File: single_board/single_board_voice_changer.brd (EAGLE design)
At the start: 58.1 x 48.2 mm, 26 parts, among them U1 ATMEGA328P_PDIP

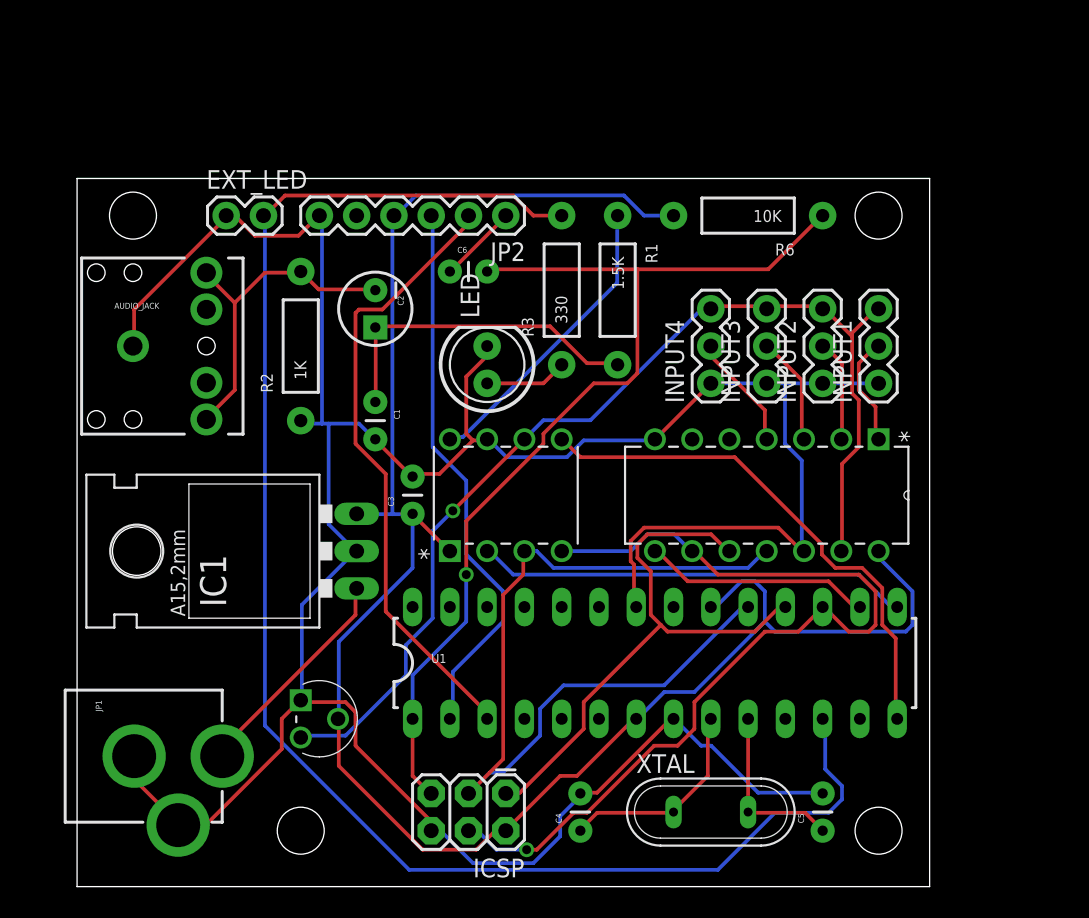
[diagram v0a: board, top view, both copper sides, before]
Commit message: board with no ground plane, 0
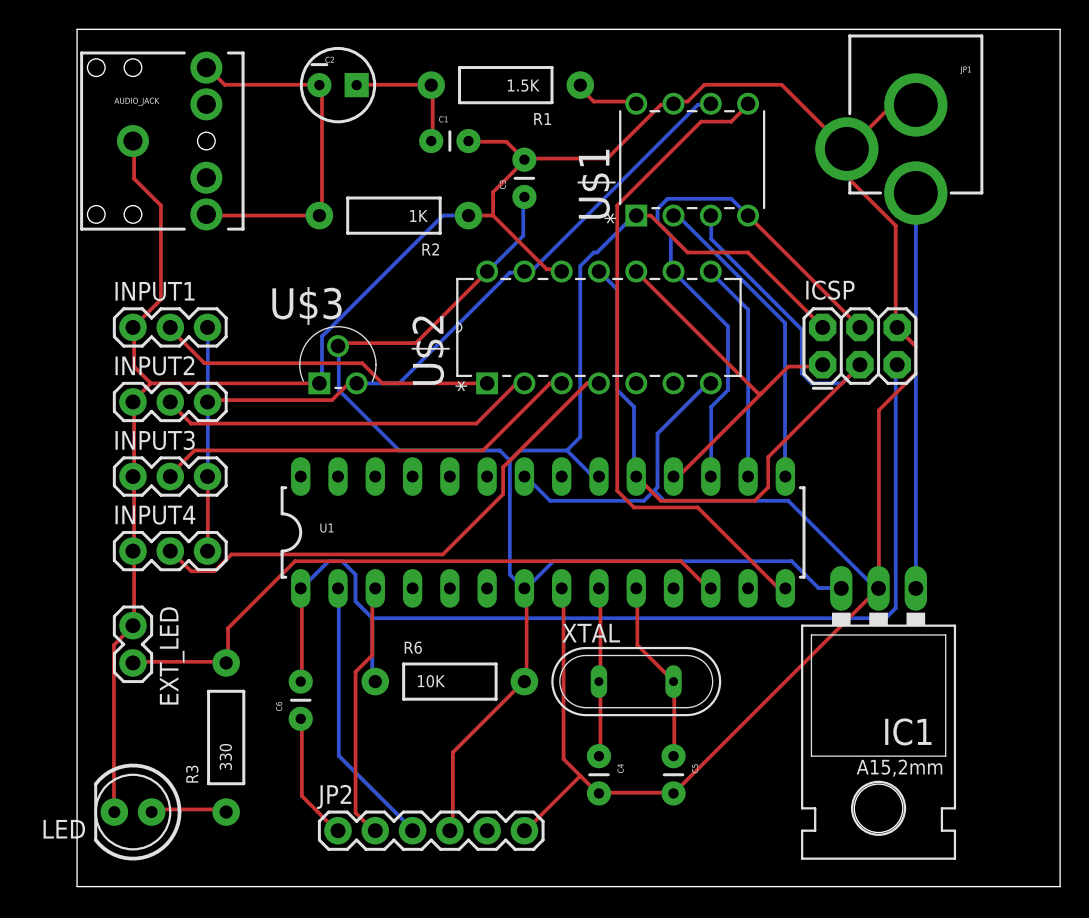
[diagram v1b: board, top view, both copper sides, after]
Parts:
- moved JP1 80.2 mm to (57.1, 61.0), turned to 180 degrees
- moved INPUT1 50.9 mm to (3.81, 38.1), turned to 0 degrees
- moved INPUT2 47.0 mm to (3.81, 33.0), turned to 0 degrees
- moved INPUT3 43.6 mm to (3.81, 27.9), turned to 0 degrees
- moved JP2 43.4 mm to (17.8, 3.81), turned to 0 degrees
- moved INPUT4 41.0 mm to (3.81, 22.9), turned to 0 degrees
- moved IC1 39.9 mm to (54.6, 16.5), turned to 180 degrees
- moved LED 38.9 mm to (3.81, 5.08), turned to 180 degrees
- moved R3 38.1 mm to (10.2, 10.2)
- moved R6 37.7 mm to (25.4, 14.0), turned to 0 degrees
- moved ICSP 36.3 mm to (50.8, 35.6), turned to 0 degrees
- moved C6 32.1 mm to (15.2, 11.4), turned to 90 degrees
- moved EXT_LED 28.7 mm to (3.81, 17.8), turned to 270 degrees
- moved U$3 26.7 mm to (19.1, 36.8), turned to 0 degrees
- moved U$1 26.2 mm to (45.7, 53.3)
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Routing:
- net LED: track 107.8 -> 44.4 mm
- net GND: track 204.3 -> 241.2 mm
- net ADC_CH3: track 7.92 -> 36.2 mm
- net TX: track 42.2 -> 17.7 mm
- net MOSI: track 62.9 -> 38.4 mm, vias 1 -> 0
- net ADC_CH2: track 7.44 -> 29.4 mm
- net RX: track 38.0 -> 18.6 mm
- net ADC_CH1: track 6.99 -> 25.9 mm
- net N$1: track 20.4 -> 4.46 mm
- net ADC_CH0: track 7.58 -> 23.2 mm
- net VREF: track 73.6 -> 58.0 mm, vias 1 -> 0
- net N$2: track 22.8 -> 8.95 mm
- net MISO: track 39.0 -> 25.4 mm
- net N$4: track 15.3 -> 26.9 mm
- net LDAC: track 35.8 -> 45.5 mm
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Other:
- board size 58.1 x 48.2 mm -> 67 x 58.4 mm

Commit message: price down to 8.77
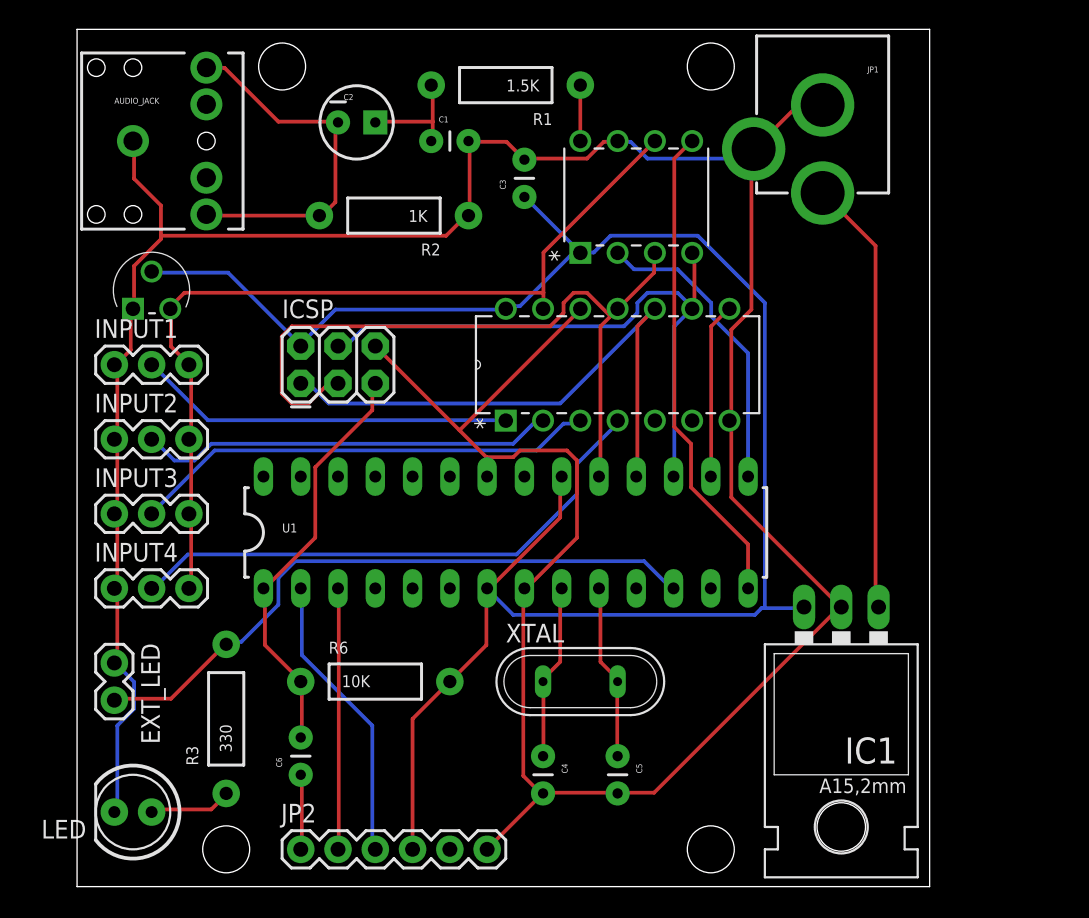
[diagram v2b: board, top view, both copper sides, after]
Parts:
- moved ICSP 35.6 mm to (15.2, 34.3)
- moved U$3 13.7 mm to (6.35, 41.9)
- moved JP1 6.35 mm to (50.8, 61.0)
- moved R6 5.08 mm to (20.3, 14.0)
- moved U$1 4.58 mm to (41.9, 50.8)
- moved C4 3.81 mm to (31.8, 8.89)
- moved C5 3.81 mm to (36.8, 8.89)
- moved XTAL 3.81 mm to (34.3, 14.0)
- moved C6 3.81 mm to (15.2, 7.62)
- moved INPUT2 2.84 mm to (2.54, 30.5)
- moved INPUT3 2.84 mm to (2.54, 25.4)
- moved EXT_LED 2.84 mm to (2.54, 15.2)
- moved JP2 2.84 mm to (15.2, 2.54)
- moved U$2 2.84 mm to (44.5, 39.4)
- moved IC1 2.84 mm to (52.1, 15.2)
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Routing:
- net RESET: track 71.7 -> 28.5 mm
- net GND: track 241.2 -> 225.3 mm
- net MISO: track 25.4 -> 39.3 mm
- net LDAC: track 45.5 -> 33.1 mm
- net MOSI: track 38.4 -> 42.5 mm
- net DTR: track 8.76 -> 5.13 mm
- net SCK: track 54.1 -> 50.8 mm
- net SS_ADC: track 15.0 -> 12.0 mm
- net N$4: track 26.9 -> 29.8 mm
- net ADC_CH2: track 29.4 -> 32.0 mm
- net VREF: track 58.0 -> 60.6 mm
- net ADC_CH1: track 25.9 -> 28.4 mm
- net ADC_CH0: track 23.2 -> 25.7 mm
- net ADC_CH3: track 36.2 -> 37.8 mm
- net RX: track 18.6 -> 19.9 mm
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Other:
- board size 67 x 58.4 mm -> 58.1 x 58.4 mm
